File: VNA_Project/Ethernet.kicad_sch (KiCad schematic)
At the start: 30 parts, among them J502 8P8C_LED_Shielded_x2, SW501 SW_SPDT, U501 LAN8742A, U502 USBLC6-4SC6, Y501 STDCZS1-25M

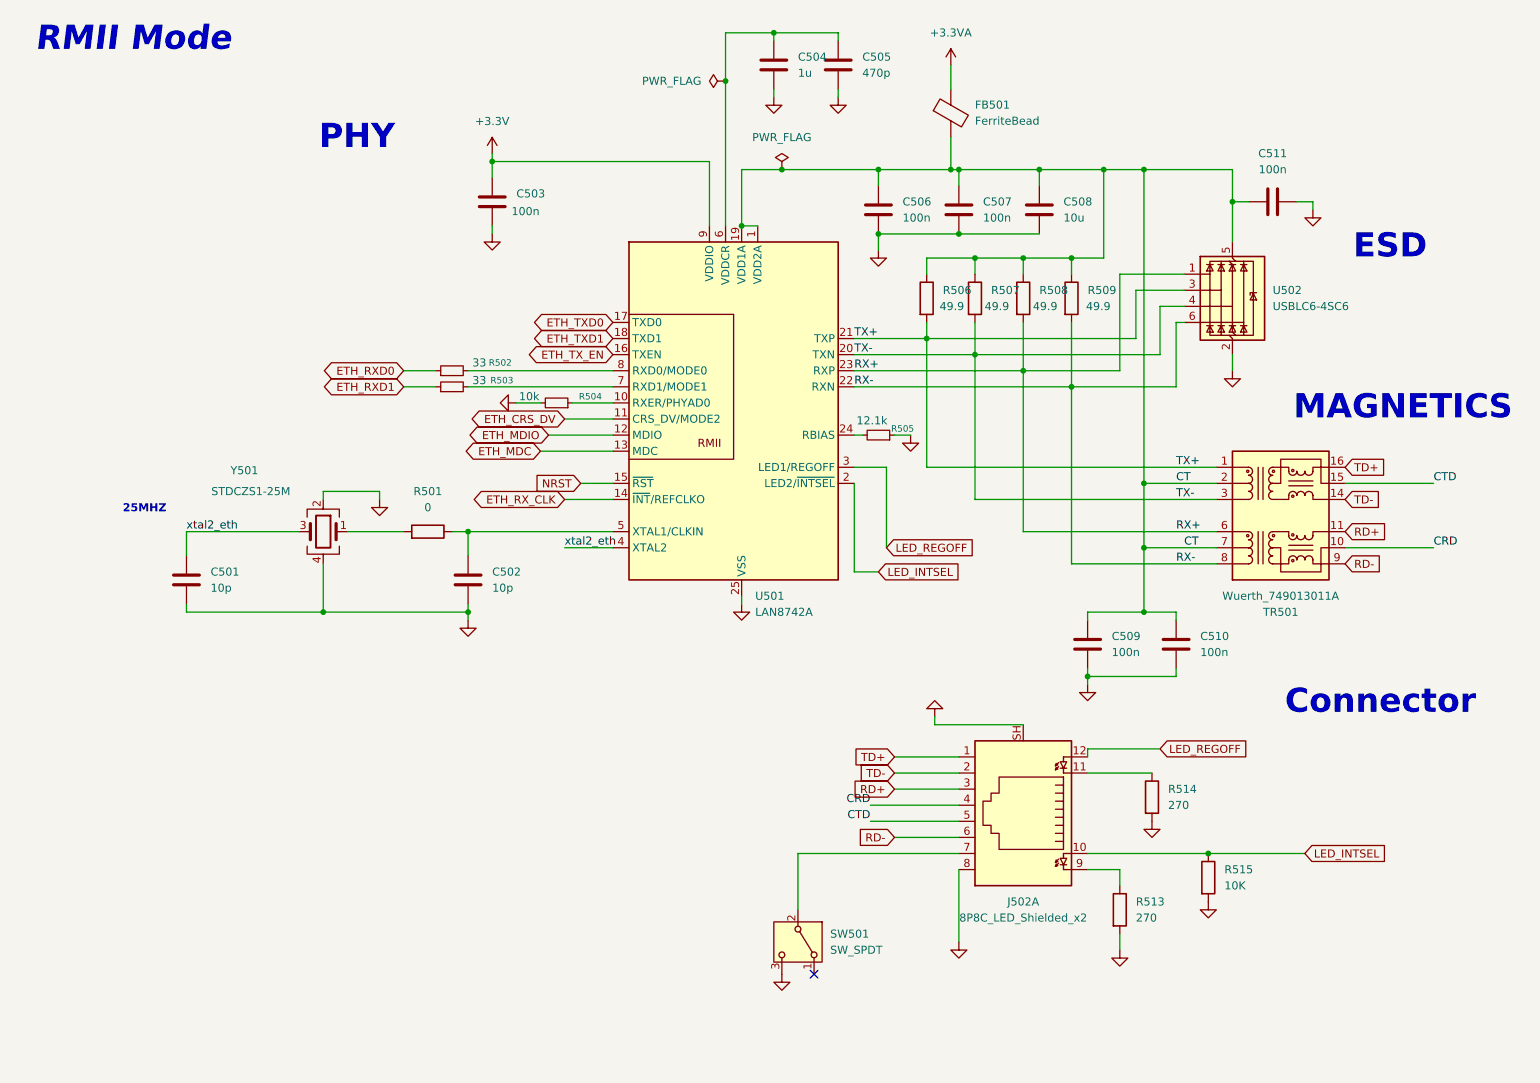
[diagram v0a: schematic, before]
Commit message: ethernet Layout
Ethernet Layout
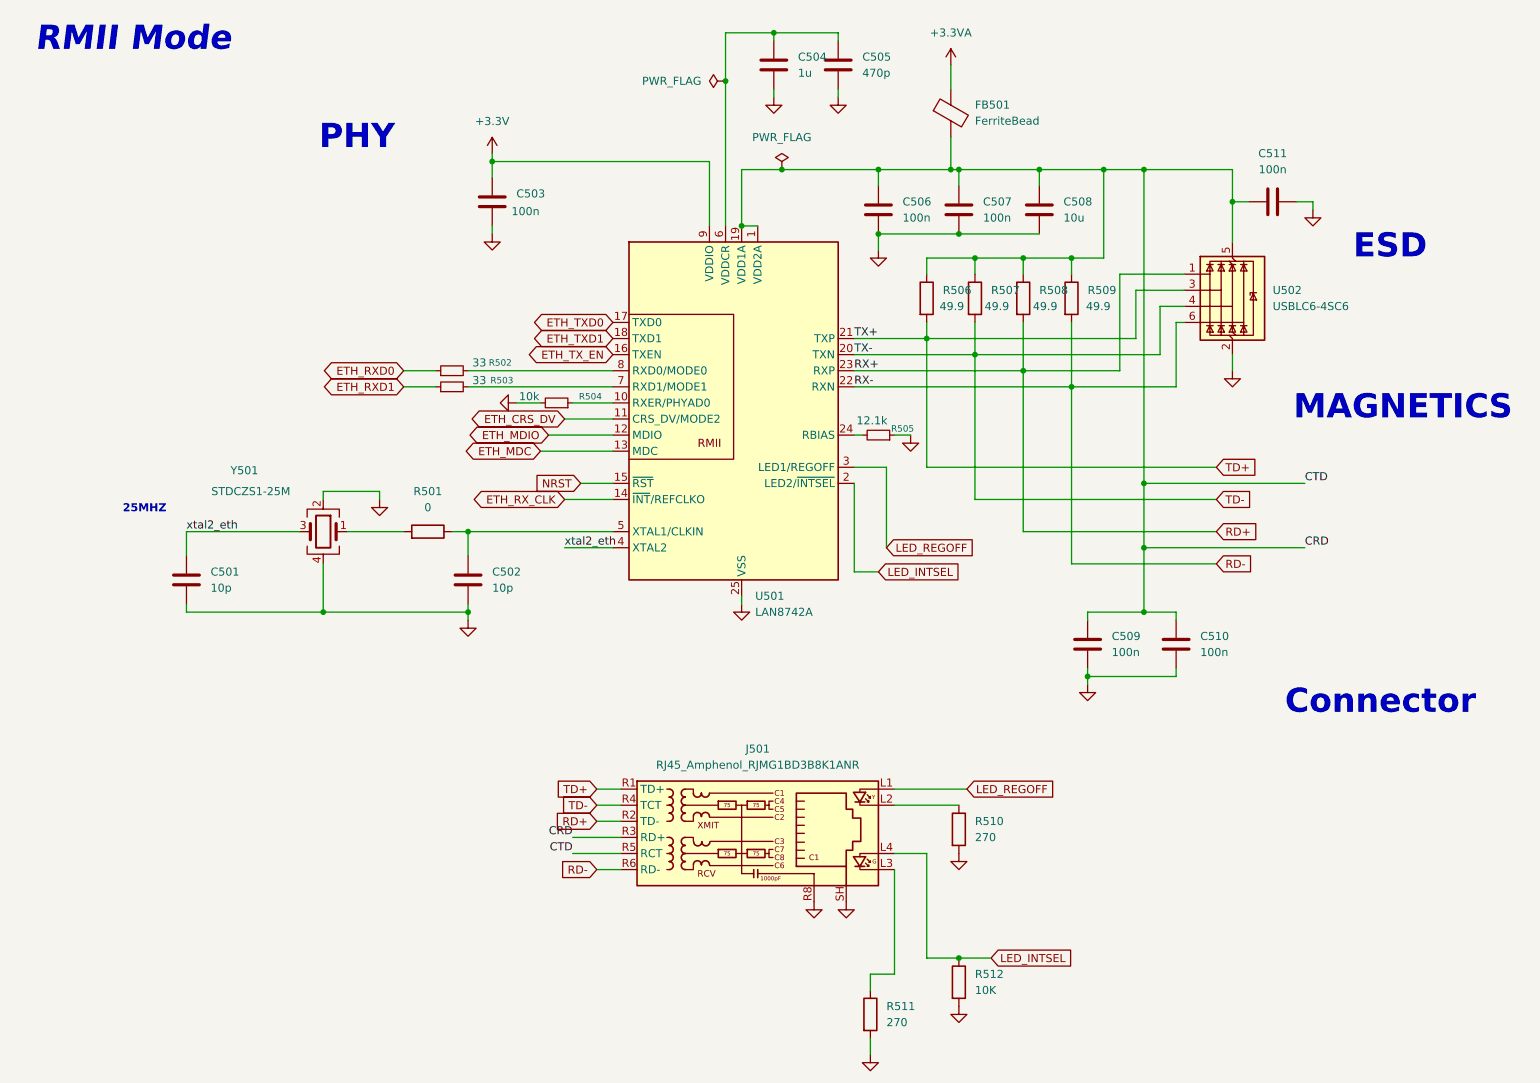
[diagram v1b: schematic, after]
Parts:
- removed J502: 8P8C_LED_Shielded_x2, Connector_RJ:RJ45_Wuerth_7499010211A_Horizontal, symbol Connector:8P8C_LED_Shielded_x2
- removed R513, R514: 270, Resistor_SMD:R_0603_1608Metric_Pad0.98x0.95mm_HandSolder, symbol Device:R
- removed R515: 10K, Resistor_SMD:R_0603_1608Metric_Pad0.98x0.95mm_HandSolder, symbol Device:R
- removed SW501: SW_SPDT, Button_Switch_THT:SW_Slide_SPDT_Straight_CK_OS102011MS2Q, symbol Switch:SW_SPDT
- removed TR501: Wuerth_749013011A, Transformer_SMD:Transformer_Ethernet_Wuerth_749013011A, symbol Transformer:Wuerth_749013011A
- added J501: RJ45_Amphenol_RJMG1BD3B8K1ANR, Connector_RJ:RJ45_Amphenol_RJMG1BD3B8K1ANR, symbol Connector:RJ45_Amphenol_RJMG1BD3B8K1ANR
- added R510, R511: 270, Resistor_SMD:R_0603_1608Metric_Pad0.98x0.95mm_HandSolder, symbol Device:R
- added R512: 10K, Resistor_SMD:R_0603_1608Metric_Pad0.98x0.95mm_HandSolder, symbol Device:R
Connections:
- net CT is gone; now on net CRD: C506.1, C507.1, C508.1, C509.1, C510.1, C511.1, FB501.2, R506.1, R507.1, R508.1, R509.1, U501.1 (VDD2A), U501.19 (VDD1A), U502.5 (VBUS)
- net RX+ is gone; now on net RD+: R508.2, U501.23 (RXP), U502.1 (I/O1)
- net RX- is gone; now on net RD-: R509.2, U501.22 (RXN), U502.6 (I/O4)
- net TX+ is gone; now on net TD+: R506.2, U501.21 (TXP), U502.3 (I/O2)
- net TX- is gone; now on net TD-: R507.2, U501.20 (TXN), U502.4 (I/O3)
- net CRD: now also J501.R3 (RD+), J501.R5 (RCT)
- net GND: now also J501.R8, J501.SH, R510.2, R511.2, R512.2
- net LED_INTSEL: now also J501.L4, R512.1
- net LED_REGOFF: now also J501.L1
- net RD+: now also J501.R2 (TD-)
- net RD-: now also J501.R6 (RD-)
- net TD+: now also J501.R1 (TD+)
- net TD-: now also J501.R4 (TCT)
- new net: J501.L2, R510.1
- new net: J501.L3, R511.1
- no-connect marks 1 -> 0
